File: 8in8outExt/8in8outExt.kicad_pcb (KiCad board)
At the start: 2 copper layers, 100.1 x 43.2 mm, 50 parts, among them P1 CONN_10X2, SW1 SPST, SW2 SPST, SW3 SPST, SW4 SPST, SW5 SPST, SW6 SPST, SW7 SPST, SW8 SPST, U1 ULN2803, U2 ULN2803

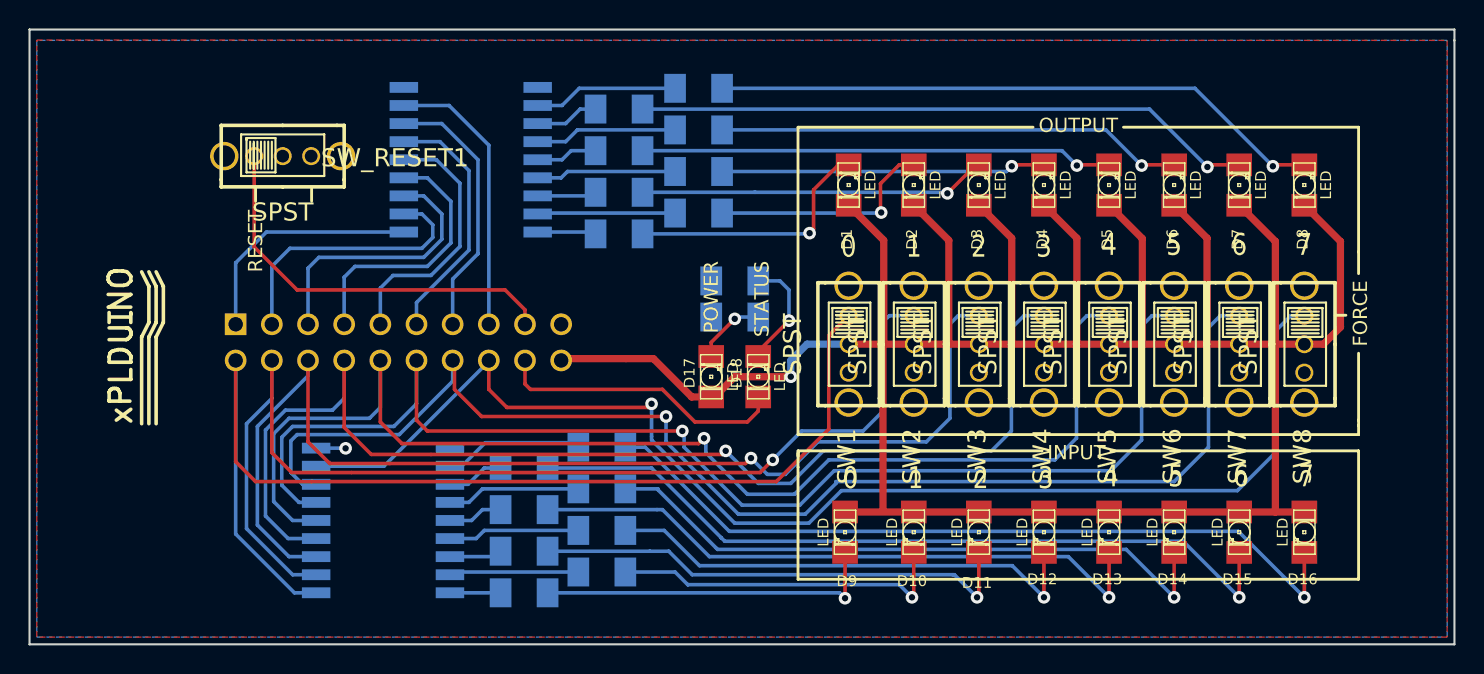
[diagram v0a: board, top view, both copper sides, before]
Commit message: mise ? jour serigraphie
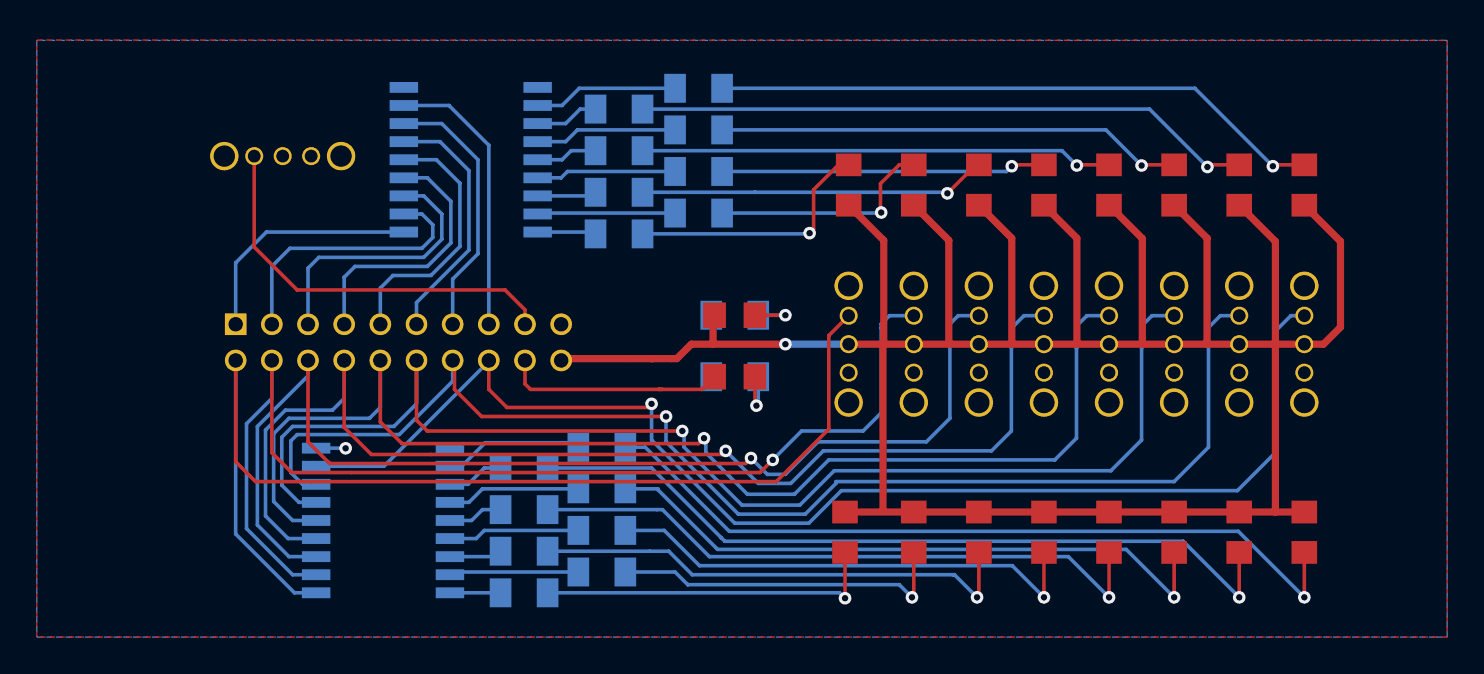
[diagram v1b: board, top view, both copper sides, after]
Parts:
- moved logo_xplduino 17.4 mm to (106.9, 107.7), turned to 0 degrees
- moved R18 6.73 mm to (135.9, 97.5)
- moved D17 4.62 mm to (135.9, 93.2), turned to 0 degrees
- moved D18 1.65 mm to (135.9, 97.5), turned to 0 degrees
- moved R17 0.13 mm to (135.9, 93.2)
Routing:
- net LED: track 20.4 -> 15.7 mm
- net N-0000028: track 7.99 -> 4.16 mm
- net N-0000030: track 5.03 -> 4.04 mm
- net +5V: track 199.8 -> 199.1 mm
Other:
- board outline removed
- board text added: "NORM"
- board text added: "NORMAL"
- board text added: "home automation"
